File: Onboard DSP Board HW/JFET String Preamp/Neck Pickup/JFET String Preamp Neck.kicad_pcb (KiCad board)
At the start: 2 copper layers, 28.4 x 89.9 mm, 41 parts, among them J1 Input, J10 Input, J14 Input, J5 Input, Q1 MMBF201, Q2 MMBF201, Q3 MMBF201, Q4 MMBF201

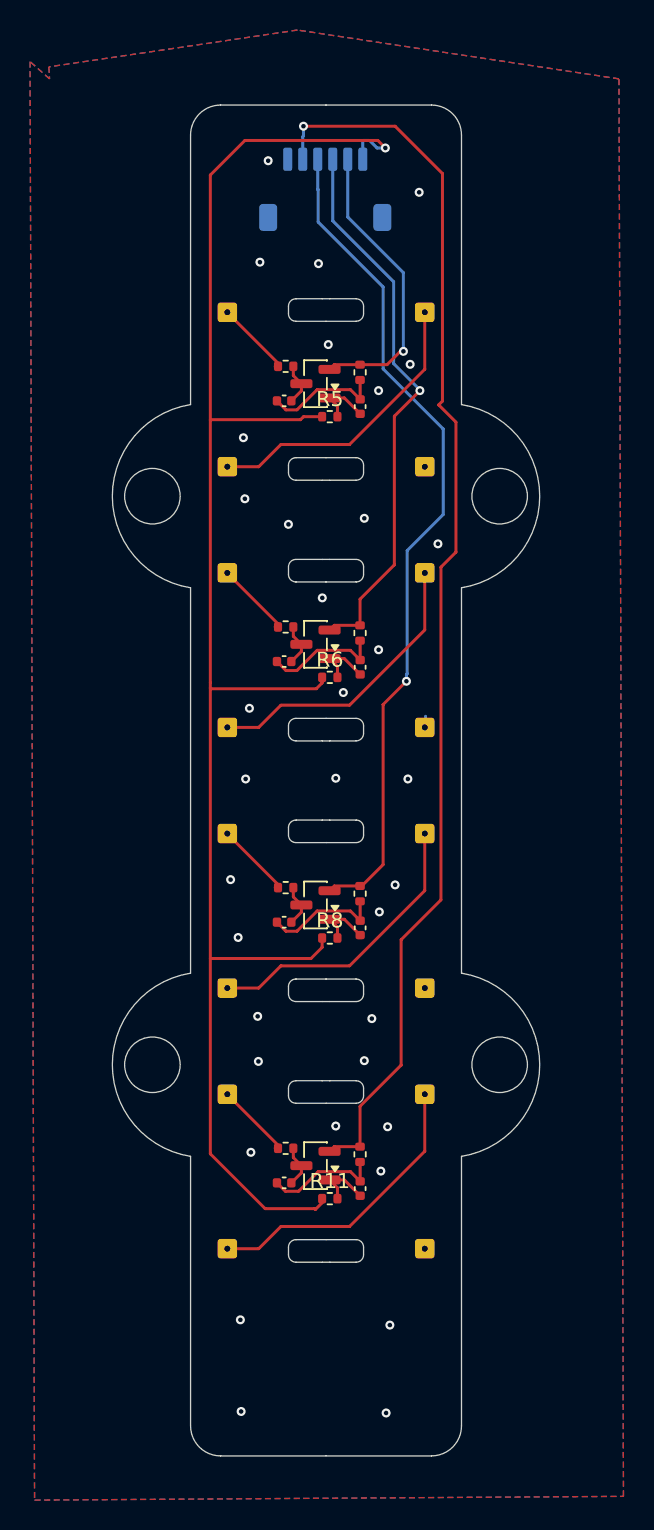
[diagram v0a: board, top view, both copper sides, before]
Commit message: WIP
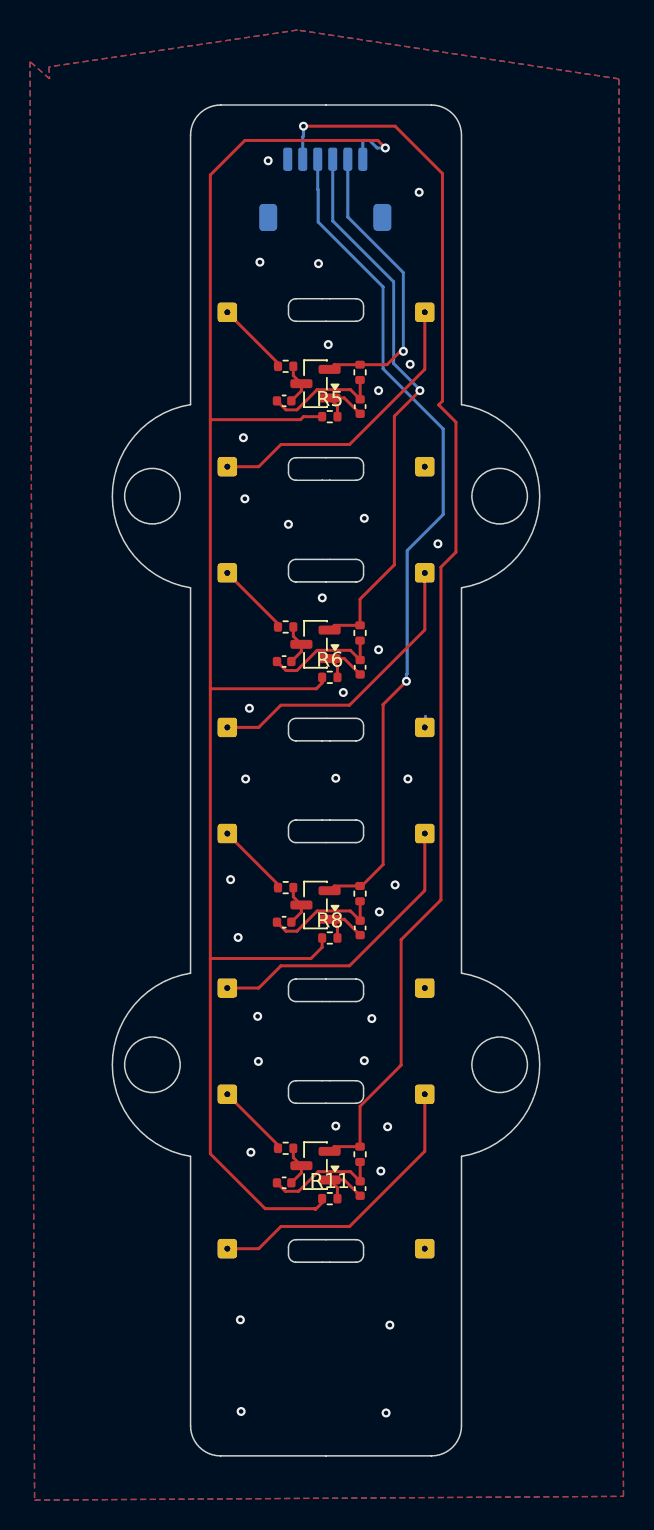
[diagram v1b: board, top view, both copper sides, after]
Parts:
- C3, C4, C6, C8: value 100nF -> 100pF
